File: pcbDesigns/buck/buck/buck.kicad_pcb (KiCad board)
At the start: 2 copper layers, 85 x 105 mm, 17 parts, among them J1 GND, J2 5V, J3 ESP_CONNECTOR, J4 RECTIFIER_IN, J5 PWM_OUT, J6 CURR_SENS, Q1 IXGH24N60C4D1, U1 TLP250

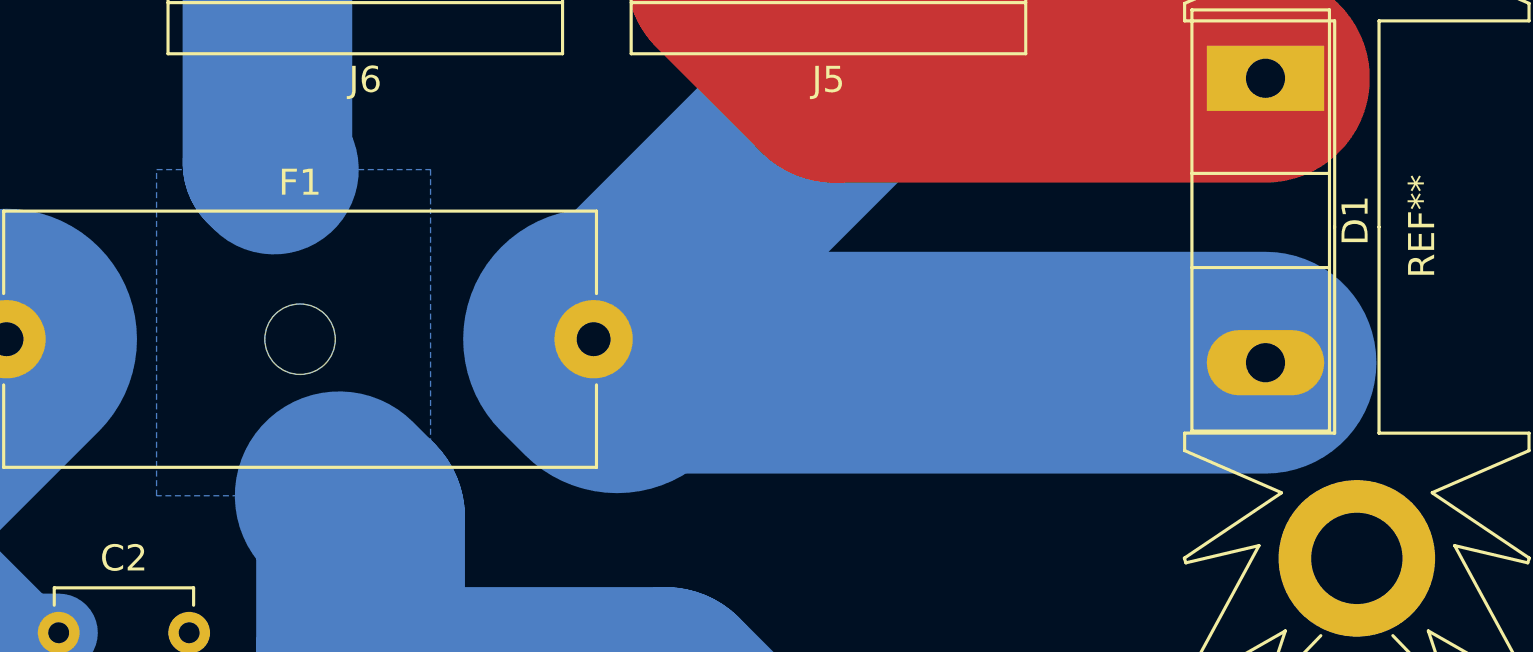
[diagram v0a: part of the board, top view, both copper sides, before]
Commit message: more revision
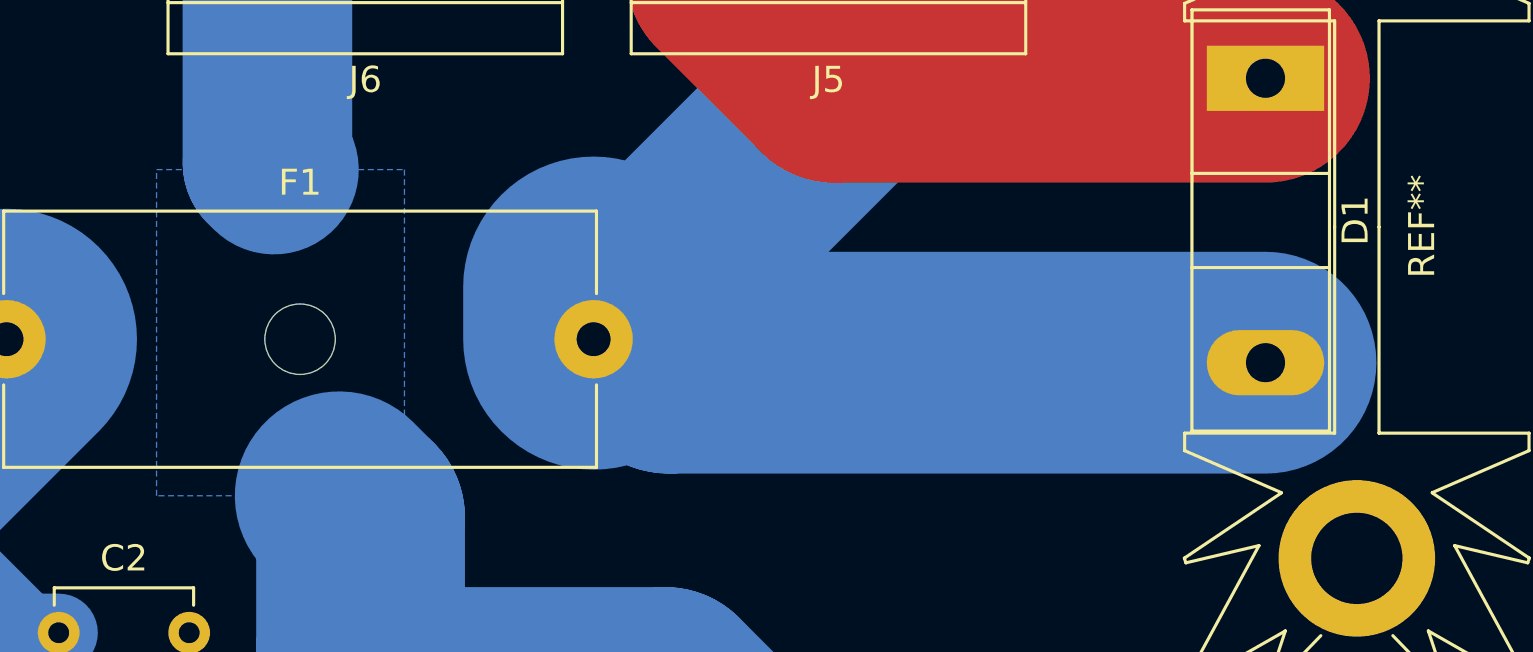
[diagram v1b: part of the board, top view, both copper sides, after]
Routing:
- net VCC: track 47.9 -> 50.7 mm
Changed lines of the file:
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@@
   (segment (start 184 54) (end 180 50) (width 8) (layer "F.Cu") (net 3))
   (segment (start 169.75 47.5) (end 180 47.5) (width 6.5) (layer "B.Cu") (net 3))
-  (segment (start 200.5 64.9) (end 175.65 64.9) (width 8.5) (layer "B.Cu") (net 4))
   (segment (start 187.5 47.5) (end 187.5 51.25) (width 8) (layer "B.Cu") (net 4))
   (segment (start 187.5 51.25) (end 174.75 64) (width 8) (layer "B.Cu") (net 4))
-  (segment (start 175.65 64.9) (end 174.75 64) (width 10) (layer "B.Cu") (net 4))
+  (segment (start 200.5 64.9) (end 177.65 64.9) (width 8.5) (layer "B.Cu") (net 4))
+  (segment (start 174.75 62) (end 174.75 64) (width 10) (layer "B.Cu") (net 4))
+  (segment (start 177.65 64.9) (end 174.75 62) (width 8.5) (layer "B.Cu") (net 4))
   (segment (start 187.0885 116.0885) (end 190.8085 119.8085) (width 2) (layer "F.Cu") (net 5))
   (segment (start 187.0885 112.6085) (end 187.0885 116.0885) (width 2) (layer "F.Cu") (net 5))
@@
     (polygon
       (pts
-        (xy 168.5 70)
+        (xy 167.5 70)
         (xy 158 70)
         (xy 158 57.5)
-        (xy 168.5 57.5)
+        (xy 167.5 57.5)
       )
     )
